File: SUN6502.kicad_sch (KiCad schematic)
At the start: 10 parts, among them SW1 RESET, U1 W65C02SxP, U2 KM62256CLP, U3 28C256, U5 74LS139, U6 74LS138, Y1 1Mhz

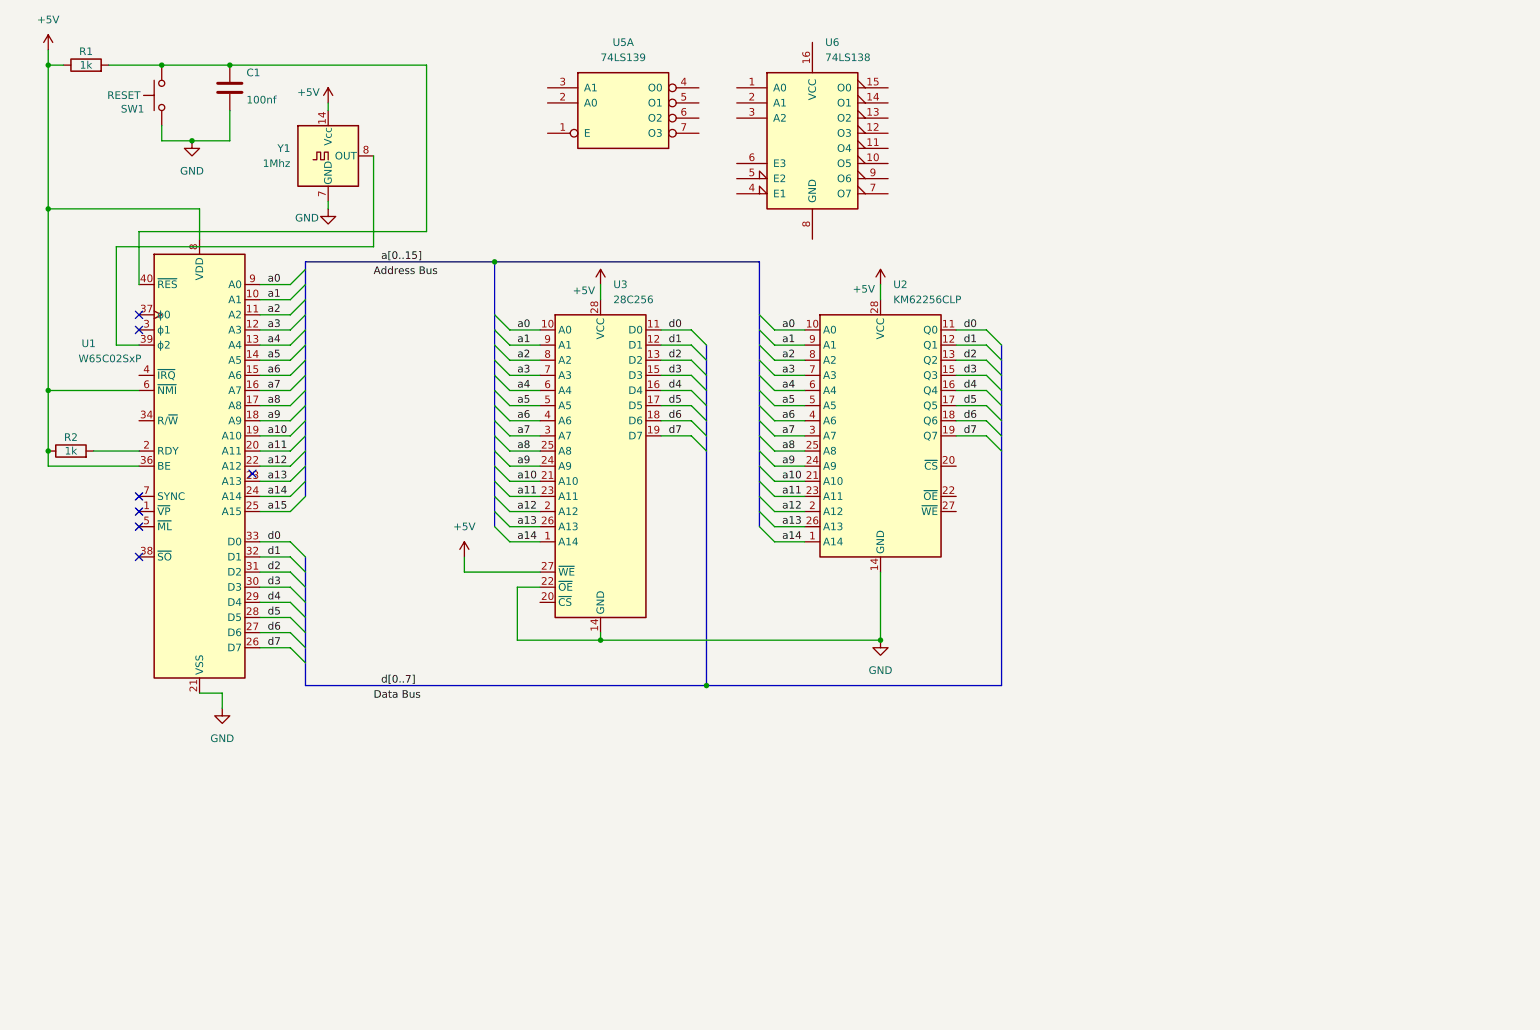
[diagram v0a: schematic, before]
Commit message: updates
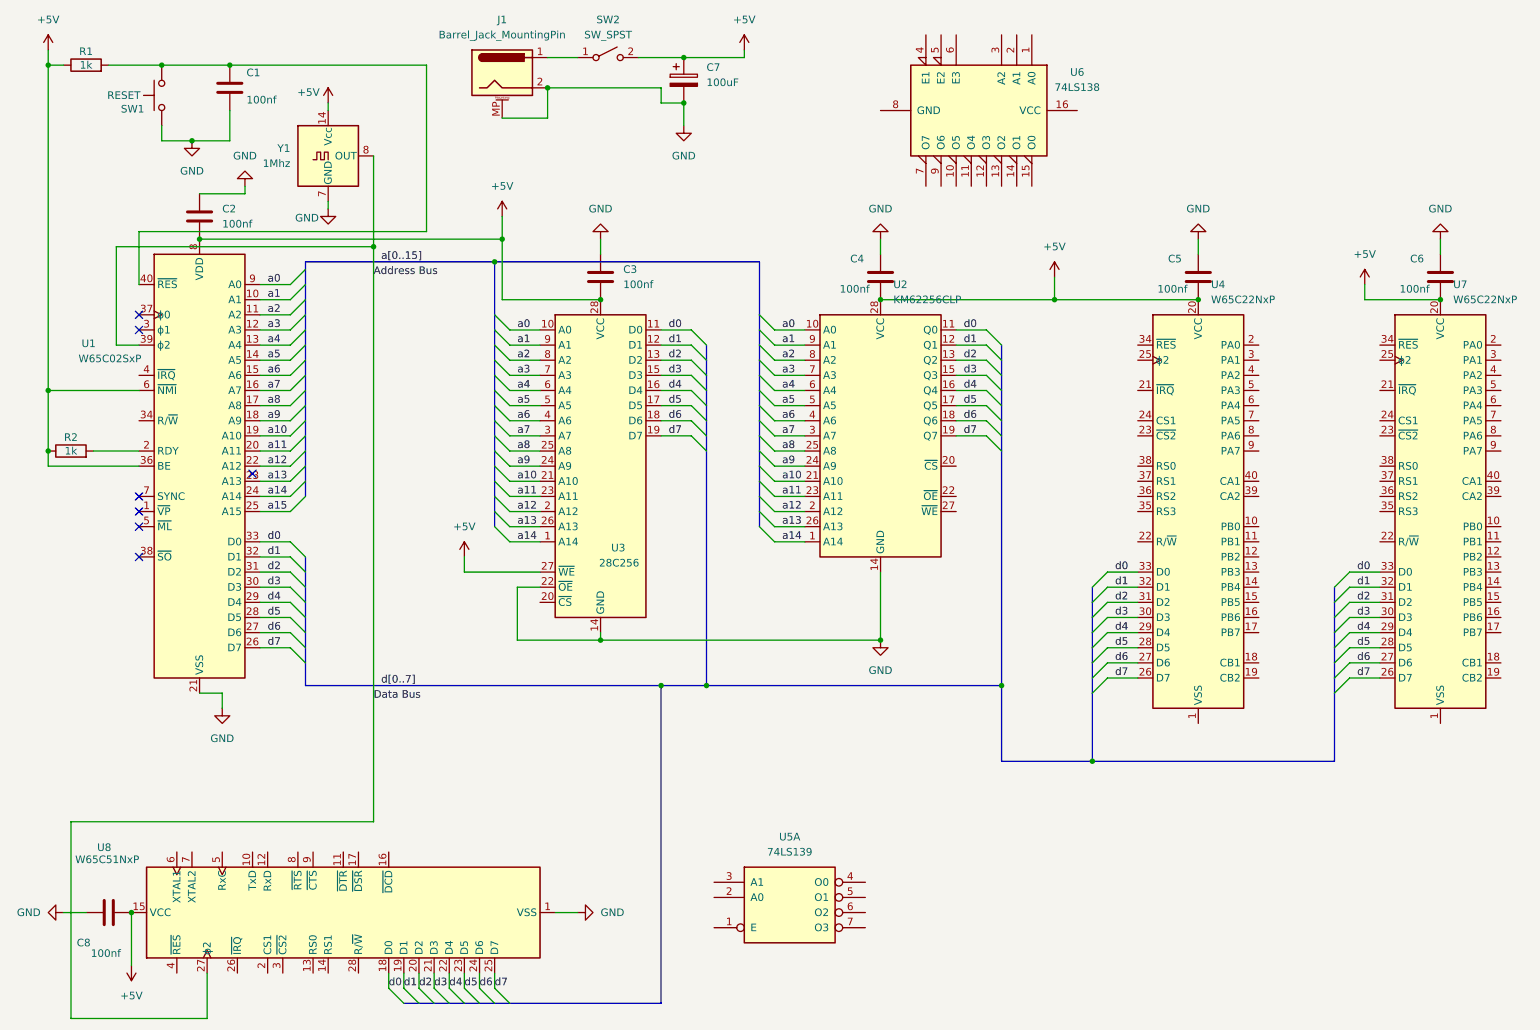
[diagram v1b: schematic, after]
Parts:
- added C2, C3, C4, C5, C6, C8: 100nf, symbol Device:C
- added C7: 100uF, symbol Device:C_Polarized
- added J1: Barrel_Jack_MountingPin, Connector_BarrelJack:BarrelJack_Horizontal, symbol Connector:Barrel_Jack_MountingPin
- added SW2: SW_SPST, symbol Switch:SW_SPST
- added U4, U7: W65C22NxP, Package_DIP:DIP-40_W15.24mm, symbol PCM_65xx-library:W65C22NxP
- added U8: W65C51NxP, Package_DIP:DIP-28_W15.24mm, symbol PCM_65xx-library:W65C51NxP
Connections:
- net +5V: now also C2.2, C3.2, C4.2, C5.2, C6.2, C7.1, C8.2, SW2.2 (B), U4.20 (VCC), U7.20 (VCC), U8.15 (VCC)
- net Address Bus: now also U1.39 (ϕ2), Y1.8 (OUT), U8.27 (ϕ2)
- net GND: now also C2.1, C3.1, C4.1, C5.1, C6.1, C7.2, C8.1, J1.2, J1.MP (MountPin), U8.1 (VSS)
- net d0: now also U4.33 (D0), U7.33 (D0), U8.18 (D0)
- net d1: now also U4.32 (D1), U7.32 (D1), U8.19 (D1)
- net d2: now also U4.31 (D2), U7.31 (D2), U8.20 (D2)
- net d3: now also U4.30 (D3), U7.30 (D3), U8.21 (D3)
- net d4: now also U4.29 (D4), U7.29 (D4), U8.22 (D4)
- net d5: now also U4.28 (D5), U7.28 (D5), U8.23 (D5)
- net d6: now also U4.27 (D6), U7.27 (D6), U8.24 (D6)
- net d7: now also U4.26 (D7), U7.26 (D7), U8.25 (D7)
- new net: J1.1, SW2.1 (A)
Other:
- company: (none) -> Wróbel Sebastian (Aktr0s)
- title: (none) -> Sun6502 Computer
- moved on the sheet: U5A, U6

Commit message: updates, removed backup files
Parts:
- removed U6: 74LS138, symbol 74xx:74LS138
- added BZ1: Buzzer, Buzzer_Beeper:Buzzer_12x9.5RM7.6, symbol Device:Buzzer
- added C10, C11, C12, C13, C9: 100nf, symbol Device:C
- added C14, C15, C16, C17: 1uF, symbol Device:C
- added D1: SB140, symbol Diode:SB140
- added D2, D3: SB140, Diode_THT:D_DO-41_SOD81_P10.16mm_Horizontal, symbol Diode:SB140
- added DS1: WC1602A, Display:WC1602A, symbol Display_Character:WC1602A
- added J2, J3: 6-5530843-5, 6-5530843-5:TE_6-5530843-5, symbol 6-5530843-5:6-5530843-5
- added J4: DE9_Socket, symbol Connector:DE9_Socket
- added R3: 1K, symbol Device:R
- added RV1: R_Potentiometer, symbol Device:R_Potentiometer
- added U10: MAX232, symbol Interface_UART:MAX232
- added unit 3 of U5
- added U6: 74LS21, symbol 74xx:74LS21
- added U9: 74LS138, symbol 74xx:74LS138
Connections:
- net +5V: now also C2.1, U4.24 (CS1), U7.24 (CS1), U8.2 (CS1), C10.2, C11.2, C12.2, C13.2, C9.2, DS1.15 (LED(+)), DS1.2 (VDD), J2.1, J2.2, U10.16 (VCC), U5.16 (VCC), U6.1, U6.14 (VCC), U9.16 (VCC); no longer C2.2
- net Address Bus: no longer U1.39 (ϕ2), U8.27 (ϕ2), Y1.8 (OUT)
- net GND: now also C2.2, U3.1 (A14), U4.1 (VSS), BZ1.2 (-), C10.1, C11.1, C12.1, C13.1, C16.2, C17.2, C9.1, DS1.1 (VSS), DS1.16 (LED(-)), J2.61, J2.62, J4.5, RV1.1, U10.15 (GND), U5.8 (GND), U6.7 (GND), U9.4 (E1), U9.5 (E2), U9.8 (GND); no longer C2.1
- net a0: now also U4.38 (RS0), U8.13 (RS0)
- net a1: now also U4.37 (RS1), U8.14 (RS1)
- net a10: now also U5.3 (A1)
- net a11: now also U5.2 (A0)
- net a12: now also U9.1 (A0)
- net a13: now also U9.2 (A1)
- net a14: now also U9.3 (A2); no longer U3.1 (A14)
- net a15: now also U2.20 (~{CS}), U2.22 (~{OE}), U9.6 (E3)
- net a2: now also U4.36 (RS2)
- net a3: now also U4.35 (RS3)
- net at C1.1, R1.2, SW1.2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: now also U4.34 (~{RES}), U7.34 (~{RES}), U8.4 (~{RES})
- net at U5.1 (E): now also U9.15 (O0)
- net at U5.4 (O0): now also U4.23 (~{CS2})
- net at U5.5 (O1): now also U7.23 (~{CS2})
- net at U5.6 (O2): now also U8.3 (~{CS2})
- net at R2.2, U1.2 (RDY): now also U1.34 (R/~{W}), U4.22 (R/~{W}), U7.22 (R/~{W}), U8.28 (R/~{W})
- net at U1.4 (~{IRQ}): now also D1.2 (A), D2.2 (A), D3.2 (A)
- net at U3.20 (~{CS}): now also U6.8
- net at U8.26 (~{IRQ}): now also D3.1 (K)
- net at U7.21 (~{IRQ}): now also D2.1 (K)
- net at U7.25 (ϕ2): now also U1.39 (ϕ2), U4.25 (ϕ2), U8.27 (ϕ2), Y1.8 (OUT)
- net at U4.10 (PB0): now also DS1.7 (D0)
- net at U4.11 (PB1): now also DS1.8 (D1)
- net at U4.12 (PB2): now also DS1.9 (D2)
- net at U4.13 (PB3): now also DS1.10 (D3)
- net at U4.14 (PB4): now also DS1.11 (D4)
- net at U4.15 (PB5): now also DS1.12 (D5)
- net at U4.16 (PB6): now also DS1.13 (D6)
- net at U4.17 (PB7): now also DS1.14 (D7)
- net at U4.2 (PA0): now also R3.1
- net at U4.21 (~{IRQ}): now also D1.1 (K)
- net at U4.7 (PA5): now also DS1.4 (RS)
- net at U4.8 (PA6): now also DS1.5 (R/W)
- net at U4.9 (PA7): now also DS1.6 (E)
- new net: J4.2, U10.14 (T1OUT)
- new net: J4.3, U10.13 (R1IN)
- new net: C16.1, U10.2 (VS+)
- new net: C15.1, U10.4 (C2+)
- new net: C15.2, U10.5 (C2-)
- new net: U6.2, U9.14 (O1)
- new net: U6.4, U9.13 (O2)
- new net: U6.5, U9.12 (O3)
- new net: C17.1, U10.6 (VS-)
- new net: C14.1, U10.1 (C1+)
- new net: C14.2, U10.3 (C1-)
- new net: BZ1.1 (+), R3.2
- new net: DS1.3 (VO), RV1.2
- new net: U6.10, U9.10 (O5)
- new net: U6.12, U9.9 (O6)
- new net: U6.13, U9.7 (O7)
- new net: U6.9, U9.11 (O4)
- no-connect marks 7 -> 27
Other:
- note added: "(CS) to Expansion Bus (Active low)"
- note added: "Unused 1K"
- moved on the sheet: C2, C3, C4, C5, C6, C7, C8, J1, R2, SW2, U1, U2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
